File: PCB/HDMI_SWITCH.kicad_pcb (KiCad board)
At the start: 4 copper layers, 37.5 x 36.5 mm, 21 parts, among them J1 HDMI_A, J2 HDMI_A, J3 HDMI_A, SW1 SW_SPDT, U1 TMDS261BPAG, U2 24LC02, U3 74HC04, U4 AMS1117-3.3

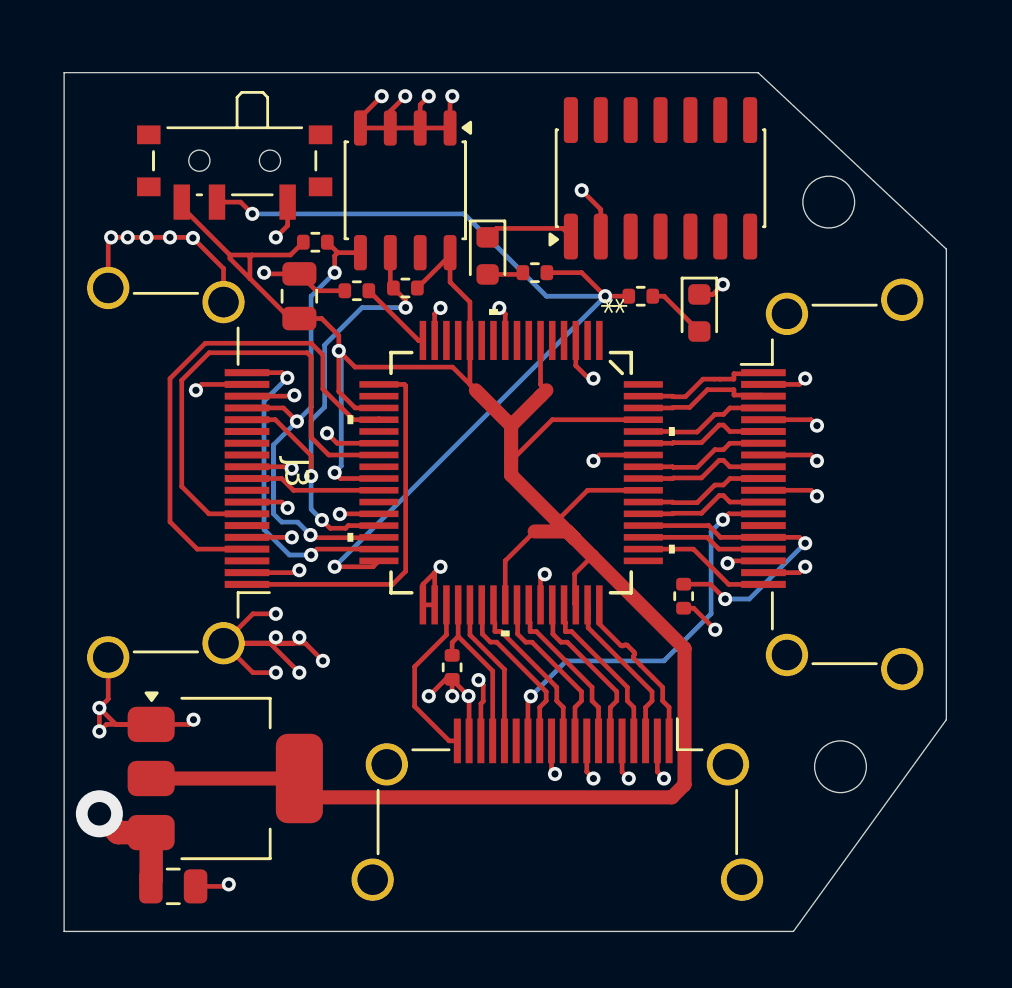
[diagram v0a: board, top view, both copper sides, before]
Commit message: Add files via upload
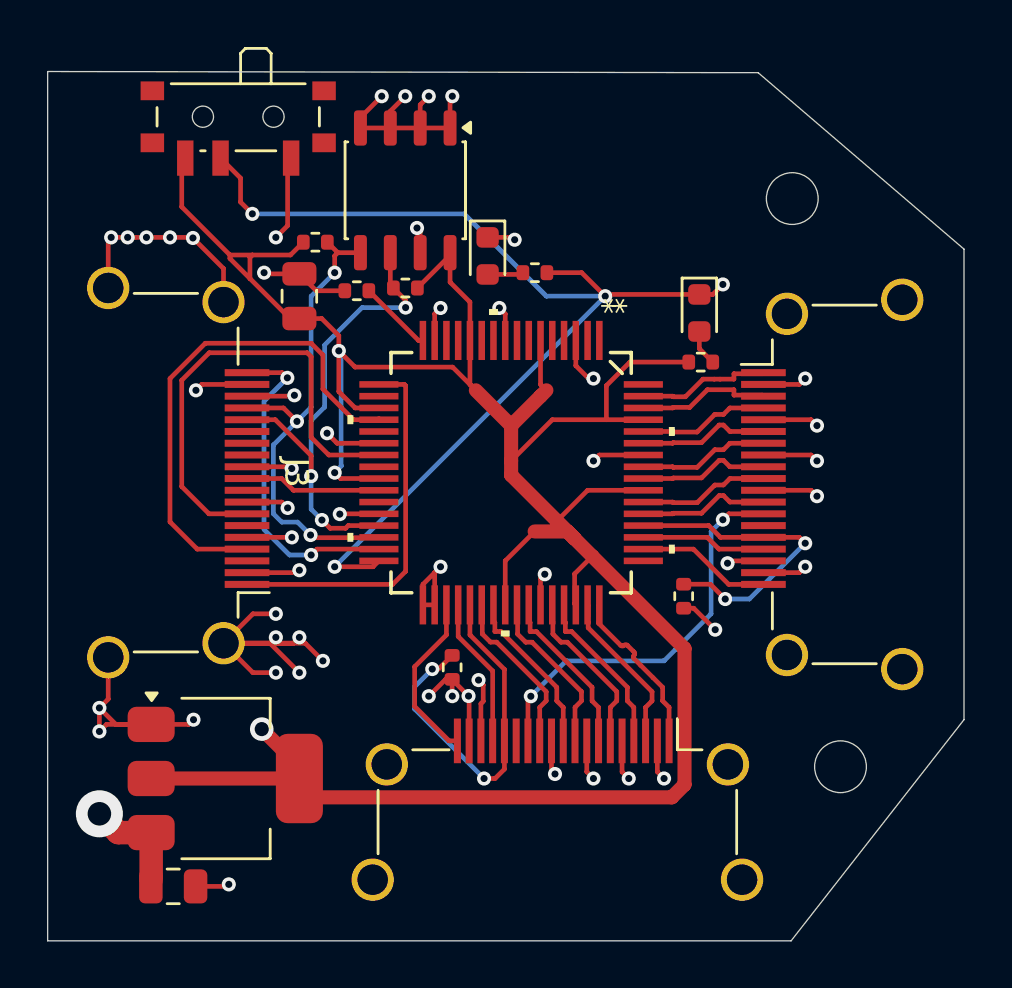
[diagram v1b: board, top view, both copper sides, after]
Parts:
- removed U3: 74HC04, Package_SO:SOIC-14_3.9x8.7mm_P1.27mm
- moved R6 3.79 mm to (129.1, 56.3), turned to 180 degrees
- moved SW1 1.88 mm to (109.4, 46.2)
- moved H2 1.56 mm to (132.9, 49.4)
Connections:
- D1 pad 1: GND -> S1
- D2 pad 1: Net-(D2-K) -> GND
- R1 pad 2: Net-(J2-SDA) -> Net-(J2-SCL)
- R6 pad 1: S1 -> Net-(D1-A)
- R6 pad 2: Net-(D1-A) -> +3.3V
- U2 pad 7: unconnected-(U2-WP-Pad7) -> GND
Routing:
- net +3.3V: track 106.6 -> 116.7 mm, vias 2 -> 3
- net Net-(J2-SCL): track 6.39 -> 15.9 mm, vias 0 -> 2
- net S1: track 40.3 -> 45.7 mm, vias 3 -> 4
- net Net-(D2-K): track 3.84 -> 0.00 mm
- net Net-(D1-A): track 2.60 -> 1.54 mm
- net GND: track 103.8 -> 104.8 mm
- net Net-(J2-SDA): track 7.30 -> 6.39 mm
- added copper zone on In2.Cu, net +3.3V
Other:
- board size 37.5 x 36.5 mm -> 39 x 37 mm
